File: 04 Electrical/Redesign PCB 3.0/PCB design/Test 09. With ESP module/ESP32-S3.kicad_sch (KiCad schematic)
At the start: 5 parts, among them U1 ESP32-S3-WROOM-1-N8R2

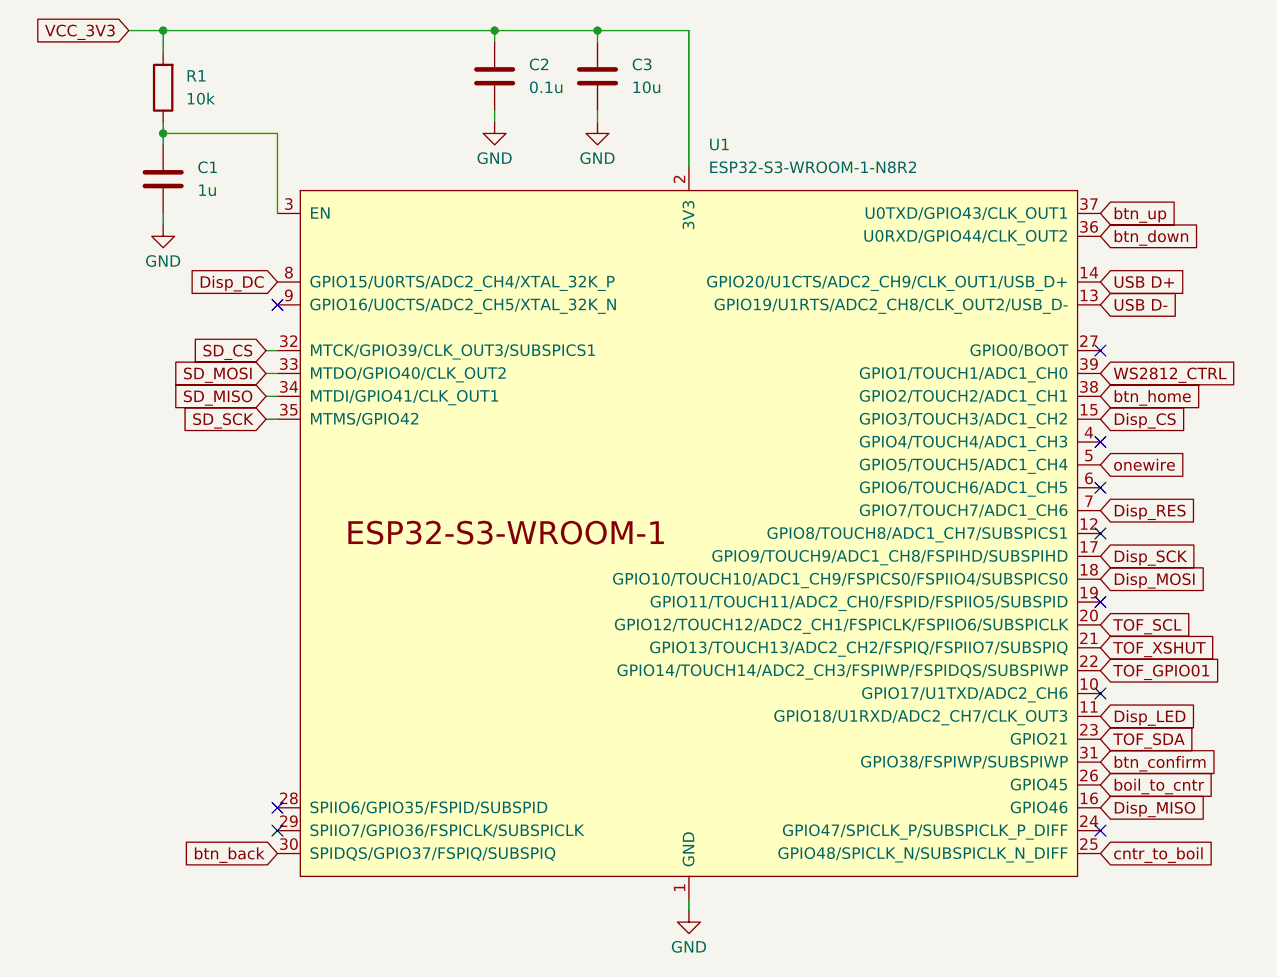
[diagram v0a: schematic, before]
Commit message: Routing PCB test 9
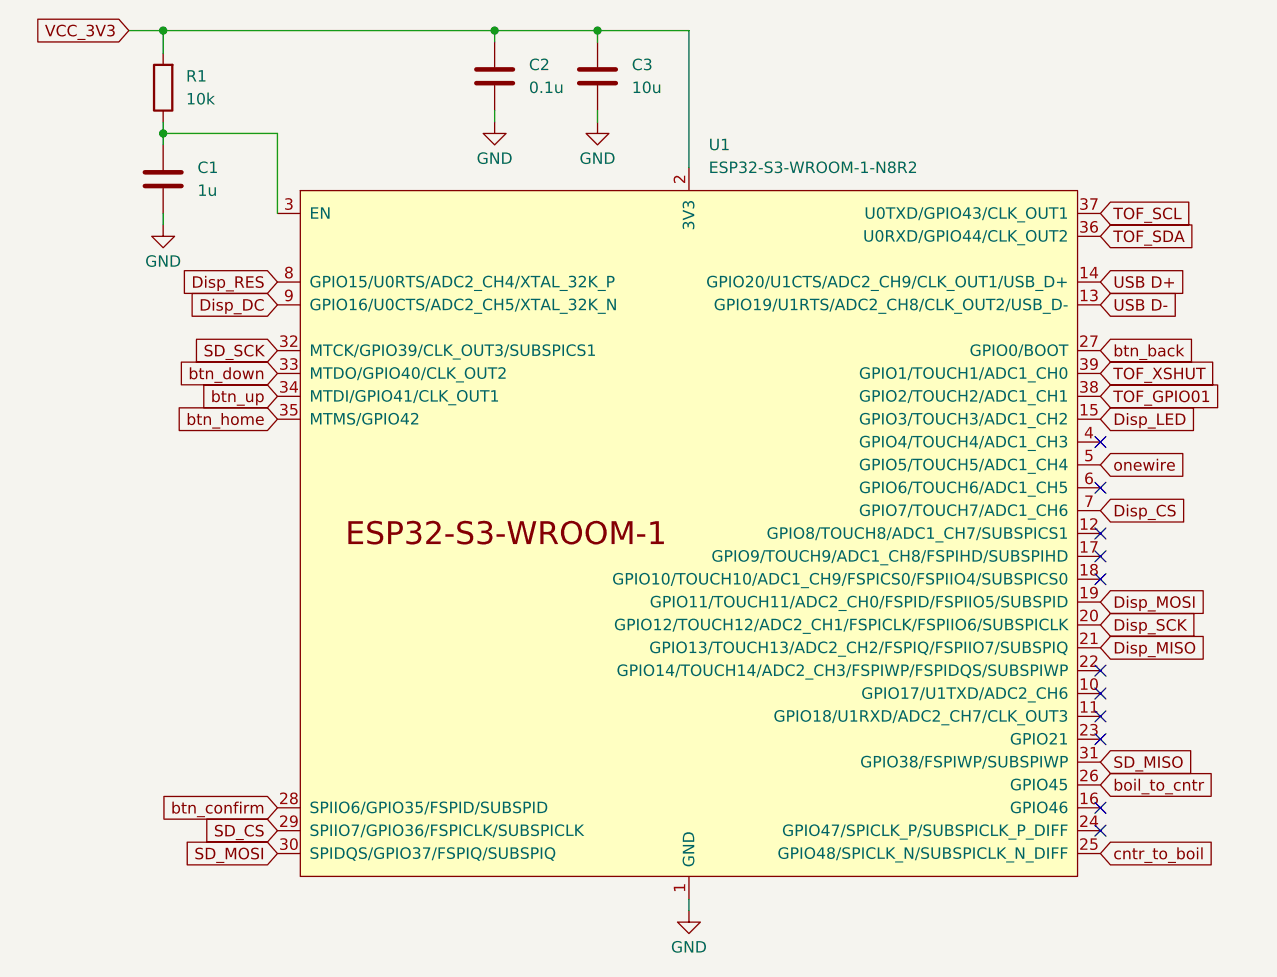
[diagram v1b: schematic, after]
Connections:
- net WS2812_CTRL is gone; now on net TOF_XSHUT: U1.39 (GPIO1/TOUCH1/ADC1_CH0)
- net Disp_CS: now also U1.7 (GPIO7/TOUCH7/ADC1_CH6); no longer U1.15 (GPIO3/TOUCH3/ADC1_CH2)
- net Disp_DC: now also U1.9 (GPIO16/U0CTS/ADC2_CH5/XTAL_32K_N); no longer U1.8 (GPIO15/U0RTS/ADC2_CH4/XTAL_32K_P)
- net Disp_LED: now also U1.15 (GPIO3/TOUCH3/ADC1_CH2); no longer U1.11 (GPIO18/U1RXD/ADC2_CH7/CLK_OUT3)
- net Disp_MISO: now also U1.21 (GPIO13/TOUCH13/ADC2_CH2/FSPIQ/FSPIIO7/SUBSPIQ); no longer U1.16 (GPIO46)
- net Disp_MOSI: now also U1.19 (GPIO11/TOUCH11/ADC2_CH0/FSPID/FSPIIO5/SUBSPID); no longer U1.18 (GPIO10/TOUCH10/ADC1_CH9/FSPICS0/FSPIIO4/SUBSPICS0)
- net Disp_RES: now also U1.8 (GPIO15/U0RTS/ADC2_CH4/XTAL_32K_P); no longer U1.7 (GPIO7/TOUCH7/ADC1_CH6)
- net Disp_SCK: now also U1.20 (GPIO12/TOUCH12/ADC2_CH1/FSPICLK/FSPIIO6/SUBSPICLK); no longer U1.17 (GPIO9/TOUCH9/ADC1_CH8/FSPIHD/SUBSPIHD)
- net SD_CS: now also U1.29 (SPIIO7/GPIO36/FSPICLK/SUBSPICLK); no longer U1.32 (MTCK/GPIO39/CLK_OUT3/SUBSPICS1)
- net SD_MISO: now also U1.31 (GPIO38/FSPIWP/SUBSPIWP); no longer U1.34 (MTDI/GPIO41/CLK_OUT1)
- net SD_MOSI: now also U1.30 (SPIDQS/GPIO37/FSPIQ/SUBSPIQ); no longer U1.33 (MTDO/GPIO40/CLK_OUT2)
- net SD_SCK: now also U1.32 (MTCK/GPIO39/CLK_OUT3/SUBSPICS1); no longer U1.35 (MTMS/GPIO42)
- net TOF_GPIO01: now also U1.38 (GPIO2/TOUCH2/ADC1_CH1); no longer U1.22 (GPIO14/TOUCH14/ADC2_CH3/FSPIWP/FSPIDQS/SUBSPIWP)
- net TOF_SCL: now also U1.37 (U0TXD/GPIO43/CLK_OUT1); no longer U1.20 (GPIO12/TOUCH12/ADC2_CH1/FSPICLK/FSPIIO6/SUBSPICLK)
- net TOF_SDA: now also U1.36 (U0RXD/GPIO44/CLK_OUT2); no longer U1.23 (GPIO21)
- net TOF_XSHUT: no longer U1.21 (GPIO13/TOUCH13/ADC2_CH2/FSPIQ/FSPIIO7/SUBSPIQ)
- net btn_back: now also U1.27 (GPIO0/BOOT); no longer U1.30 (SPIDQS/GPIO37/FSPIQ/SUBSPIQ)
- net btn_confirm: now also U1.28 (SPIIO6/GPIO35/FSPID/SUBSPID); no longer U1.31 (GPIO38/FSPIWP/SUBSPIWP)
- net btn_down: now also U1.33 (MTDO/GPIO40/CLK_OUT2); no longer U1.36 (U0RXD/GPIO44/CLK_OUT2)
- net btn_home: now also U1.35 (MTMS/GPIO42); no longer U1.38 (GPIO2/TOUCH2/ADC1_CH1)
- net btn_up: now also U1.34 (MTDI/GPIO41/CLK_OUT1); no longer U1.37 (U0TXD/GPIO43/CLK_OUT1)
- no-connect marks 10 -> 11
